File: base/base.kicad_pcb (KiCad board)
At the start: 2 copper layers, 13 parts, among them J1 Screw_Terminal_01x02, J2 Screw_Terminal_01x03, U1 CRE1S1205SC, U2 NRF24L01_Breakout

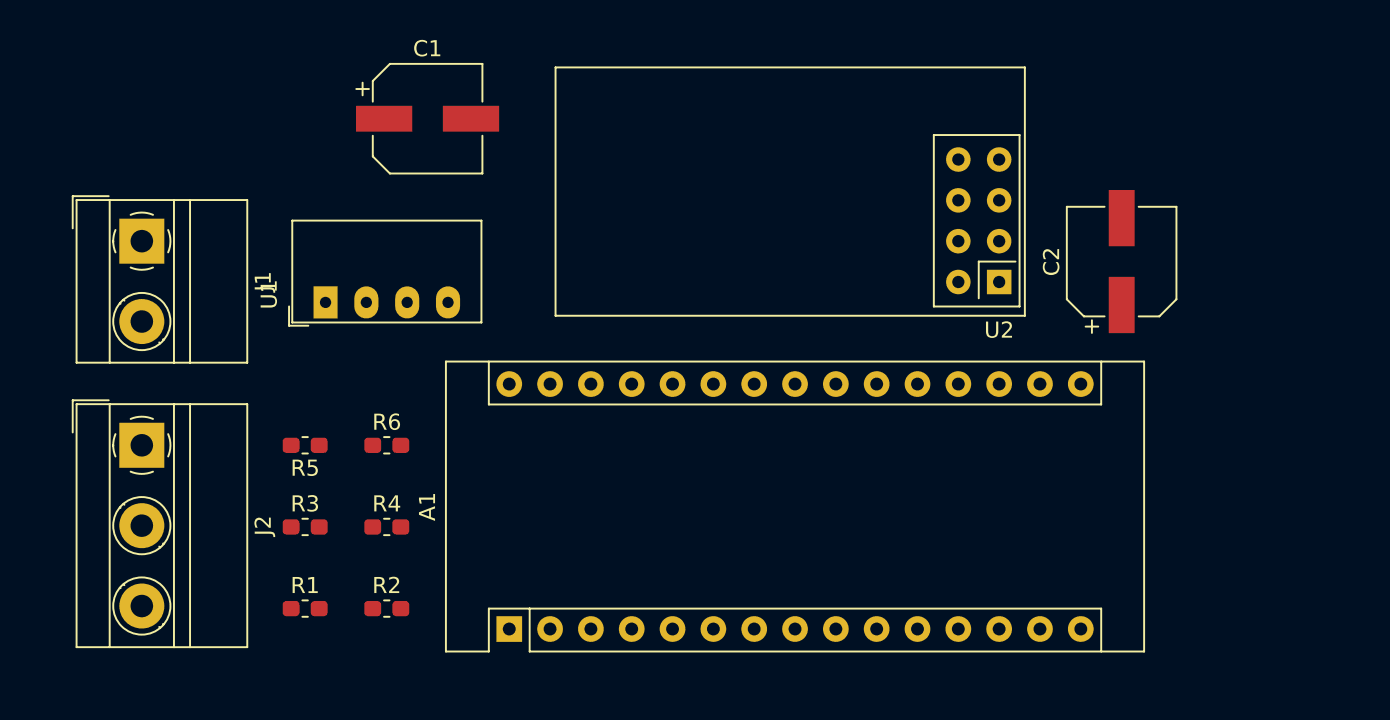
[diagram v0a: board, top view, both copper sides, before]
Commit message: Base - Lay out PCB
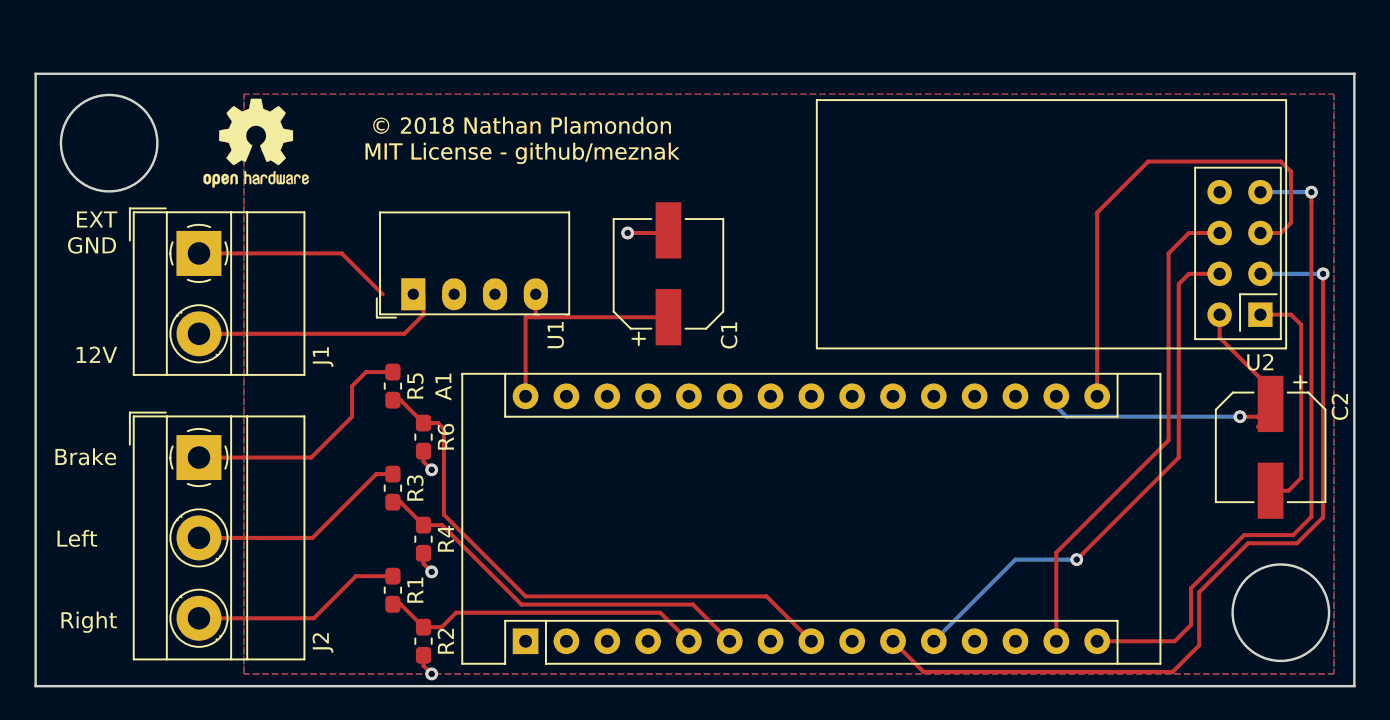
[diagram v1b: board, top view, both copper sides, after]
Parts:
- added REF**: OSHW-Logo2_7.3x6mm_Copper, Symbol:OSHW-Logo2_7.3x6mm_Copper, F.Cu at (69.3, 47.2)
- added REF**: OSHW-Logo2_7.3x6mm_SilkScreen, Symbol:OSHW-Logo2_7.3x6mm_SilkScreen, F.Cu at (69.3, 47.2)
- J1: value Screw_Terminal_01x02 -> Power
- J2: value Screw_Terminal_01x03 -> Signal
- moved C1 17.8 mm to (95.0, 55.4), turned to 90 degrees
- moved U2 16.4 mm to (131.8, 57.9)
- moved C2 14.8 mm to (132.5, 66.2), turned to 270 degrees
- moved R5 6.59 mm to (77.9, 62.4), turned to 270 degrees
- moved R3 5.97 mm to (77.9, 68.7), turned to 270 degrees
- moved R1 5.58 mm to (77.9, 75.1), turned to 270 degrees
- moved U1 5.48 mm to (79.1, 56.6)
- moved J2 3.64 mm to (65.8, 66.8)
- moved J1 3.64 mm to (65.8, 54.1)
- moved R2 3.06 mm to (79.8, 78.2), turned to 270 degrees
- moved R4 2.41 mm to (79.8, 71.9), turned to 270 degrees
- moved R6 2.34 mm to (79.8, 65.5), turned to 270 degrees
- moved A1 1.27 mm to (86.1, 78.2)
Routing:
- net Net-(A1-Pad10): track 0.00 -> 52.5 mm, vias 0 -> 1
- net Net-(A1-Pad15): track 0.00 -> 41.3 mm, vias 0 -> 1
- net Net-(A1-Pad8): track 0.00 -> 35.4 mm
- net Net-(A1-Pad11): track 0.00 -> 33.6 mm, vias 0 -> 1
- net Net-(A1-Pad14): track 0.00 -> 30.7 mm
- net Net-(A1-Pad16): track 0.00 -> 30.4 mm
- net Net-(A1-Pad6): track 0.00 -> 24.5 mm
- net +3V3: track 0.00 -> 23.5 mm, vias 0 -> 1
- net GND: track 0.00 -> 20.6 mm, vias 0 -> 4
- net Net-(A1-Pad5): track 0.00 -> 20.1 mm
- net +12V: track 0.00 -> 15.7 mm
- net Net-(J2-Pad1): track 0.00 -> 15.4 mm
- net +5V: track 0.00 -> 15.2 mm
- net Net-(J2-Pad2): track 0.00 -> 13.8 mm
- net Net-(J2-Pad3): track 0.00 -> 13.4 mm
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- added copper zone on B.Cu, net GND
- added copper zone on F.Cu, net GND
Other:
- board outline added: 82 x 38.1 mm
- board text added: "12V"
- board text added: "Brake"
- board text added: "EXT GND"
- board text added: "Left"
- board text added: "Right"
- board text added: "© 2018 Nathan Plamondon MIT License - github/meznak"

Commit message: Base - Clean up and EDC
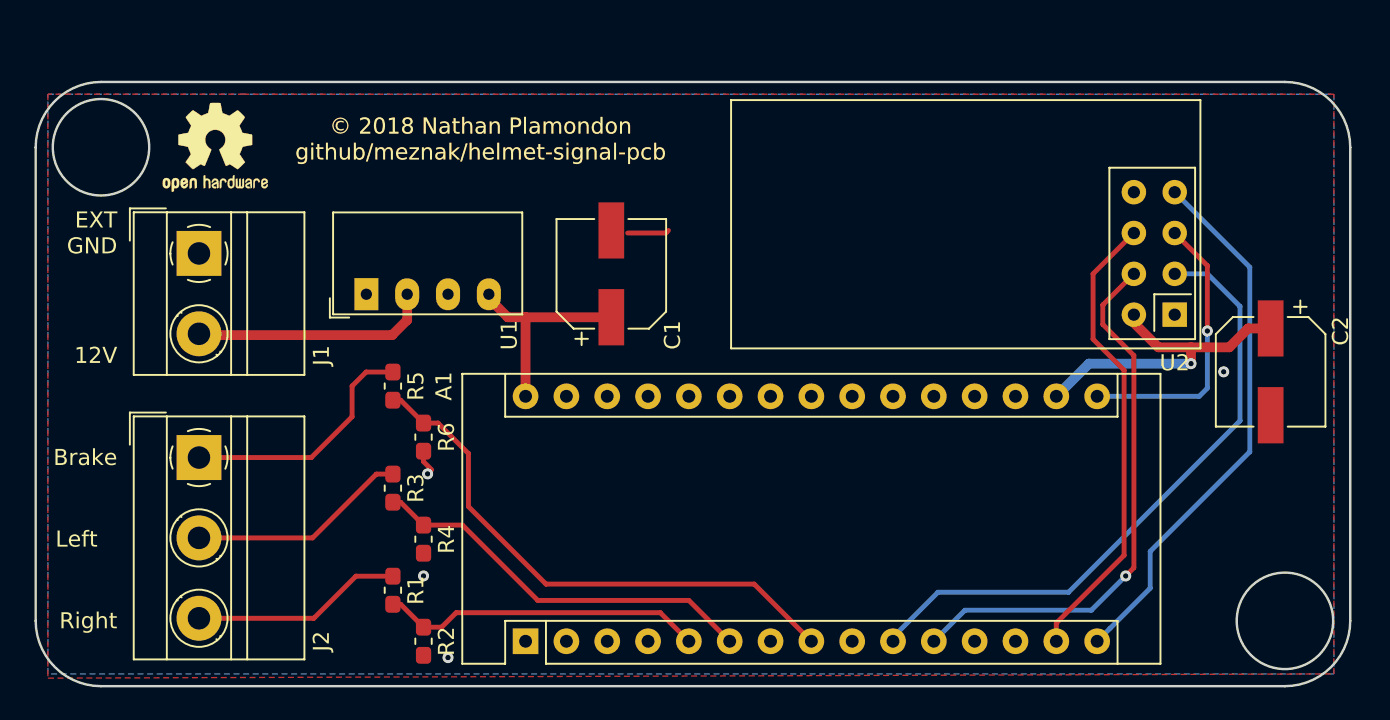
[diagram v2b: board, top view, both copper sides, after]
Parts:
- J1: value Power -> Screw_Terminal_01x02
- J2: value Signal -> Screw_Terminal_01x03
- moved U2 5.33 mm to (126.5, 57.9)
- moved C2 4.70 mm to (132.5, 61.5)
- moved C1 3.56 mm to (91.4, 55.4)
- moved U1 2.92 mm to (76.2, 56.6)
- moved REF** 2.55 mm to (66.8, 47.5) (x2)
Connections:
- J1 pad 1: GNDREF -> GND
- U1 pad 1: GNDREF -> GND
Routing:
- net GND: track 20.6 -> 4.17 mm
- net Net-(A1-Pad16): track 30.4 -> 17.6 mm, vias 0 -> 1
- net Net-(A1-Pad10): track 52.5 -> 39.8 mm, vias 1 -> 0
- net GNDREF: track 12.5 -> 0.00 mm
- net Net-(A1-Pad15): track 41.3 -> 33.8 mm, vias 1 -> 0
- net +3V3: track 23.5 -> 21.0 mm
- net +5V: track 15.2 -> 13.3 mm
- net Net-(A1-Pad14): track 30.7 -> 29.0 mm
- net Net-(A1-Pad8): track 35.4 -> 34.2 mm
- net +12V: track 15.7 -> 15.0 mm
- net Net-(A1-Pad11): track 33.6 -> 34.2 mm
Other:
- board size 82 x 38.1 mm -> 81.8 x 37.6 mm
- net class Default: clearance 0.2 -> 0.3048; trace_width 0.25 -> 0.3048; via_dia 0.8 -> 0.6858; via_drill 0.4 -> 0.3302
- net class LV Power added: clearance 0.6096, trace_width 0.6096, via_dia 0.6858, via_drill 0.3302
- net class OSHPark added: clearance 0.1524, trace_width 0.1524, via_dia 0.6858, via_drill 0.3302
- rule pad_to_mask_clearance: 0.2 -> 0.0508
- rule trace_clearance: 0.2 -> 0.3048
- rule trace_min: 0.2 -> 0.1524
- rule via_min_drill: 0.3 -> 0.254
- rule via_min_size: 0.4 -> 0.508
- board text added: "© 2018 Nathan Plamondon github/meznak/helmet-signal-pcb"
- board text removed: "© 2018 Nathan Plamondon MIT License - github/meznak"
